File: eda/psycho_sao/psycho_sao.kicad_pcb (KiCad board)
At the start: 2 copper layers, 80.2 x 117.1 mm, 21 parts

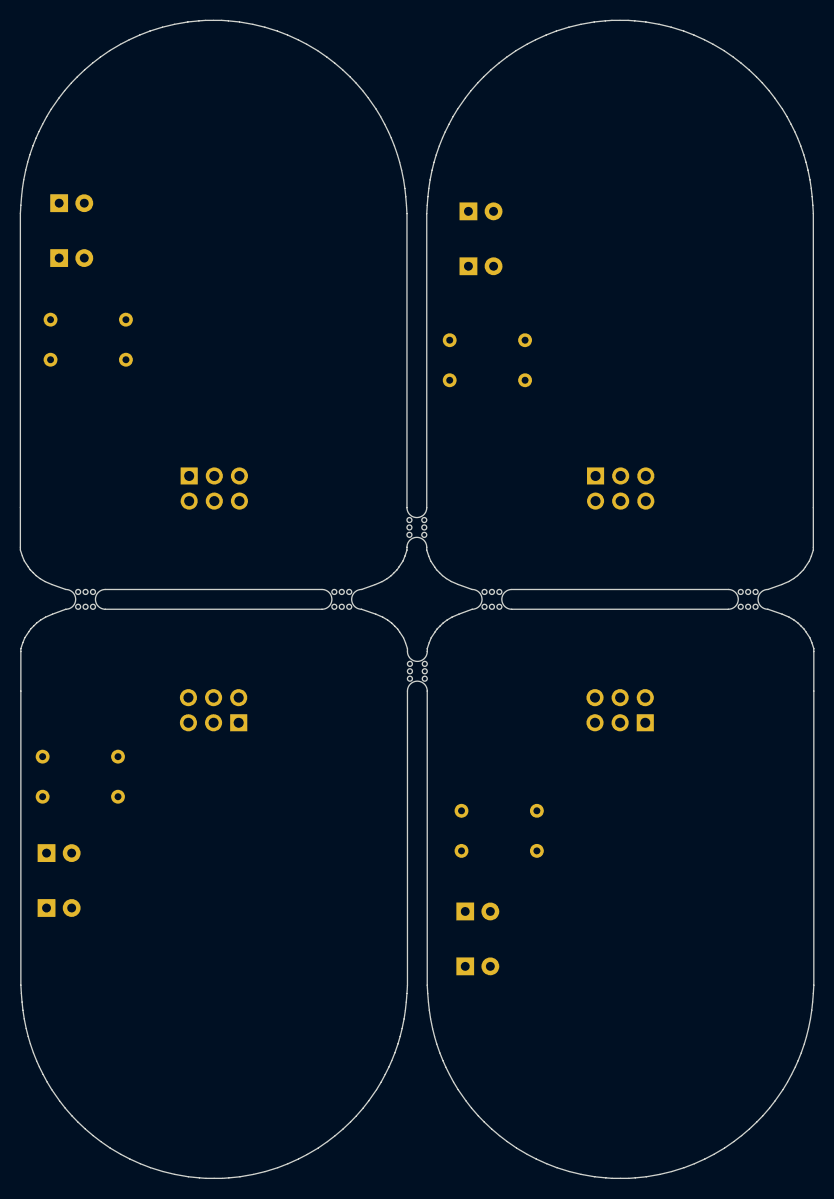
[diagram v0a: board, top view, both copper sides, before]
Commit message: psycho sao scream done
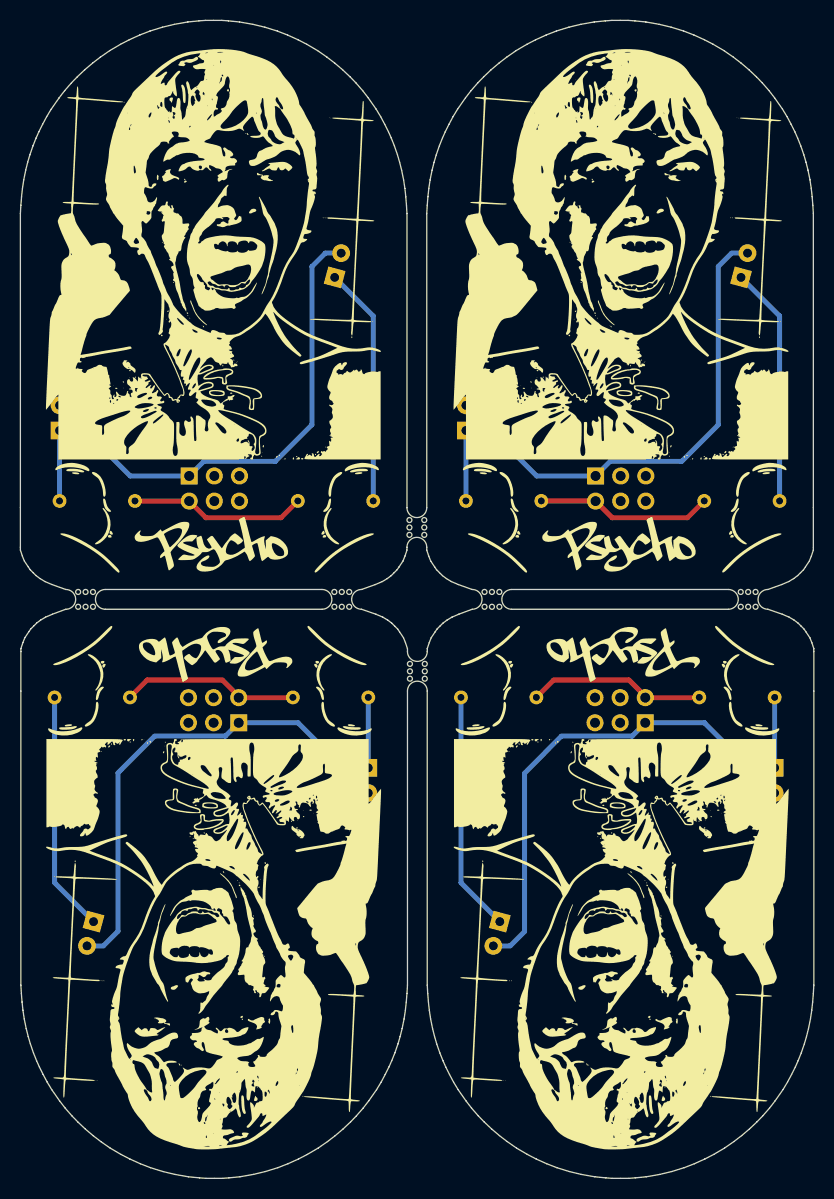
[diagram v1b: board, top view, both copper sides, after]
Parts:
- added Psycho_BMask: Psycho_BMask, 0_badge:Scream_Face_B_Mask, F.Cu at (122.1, 92.7)
- added Psycho_FCu: Psycho_FCu, 0_badge:Scream_Face_F_Cu, F.Cu at (122.1, 92.7)
- added Psycho_FMask: Psycho_FMask, 0_badge:Scream_Face_F_Mask, F.Cu at (122.1, 92.7)
- added Psycho_FSilk: Psycho_FSilk, 0_badge:Scream_Face_F_Silk, F.Cu at (122.1, 92.7)
- JSAO1, JSAO2, JSAO3, JSAO4: footprint 0_sao_v169bis:SAOv169-SAOv3-2x3 -> 0_sao_v169bis:SAOv169-SAOv3-2x3_po
- moved R12 35.6 mm to (116.1, 86.8), turned to 180 degrees
- moved R22 35.5 mm to (157.2, 86.8), turned to 180 degrees
- moved D41 34.5 mm to (156.7, 113.8), turned to -90 degrees
- moved R41 33.7 mm to (156.7, 106.7), turned to 180 degrees
- moved D31 33.6 mm to (115.6, 113.8), turned to -90 degrees
- moved R31 33.5 mm to (115.6, 106.7), turned to 180 degrees
- moved D12 27.9 mm to (112.2, 64.2), turned to 75 degrees
- moved D22 27.6 mm to (153.3, 64.2), turned to 75 degrees
- moved D11 23.0 mm to (84.4, 79.7), turned to 90 degrees
- moved D21 22.2 mm to (125.5, 79.7), turned to 90 degrees
- moved R11 18.3 mm to (84.4, 86.8)
- moved R21 16.3 mm to (125.5, 86.8)
- moved R42 15.5 mm to (125.0, 106.7)
- moved R32 10.1 mm to (83.9, 106.7)
- moved D42 5.72 mm to (128.9, 129.3), turned to -105 degrees
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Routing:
- net +3.3V: track 0.00 -> 50.1 mm
- net +3.3V1: track 0.00 -> 50.1 mm
- net +3.3V3: track 0.00 -> 50.1 mm
- net +3.3V2: track 0.00 -> 50.1 mm
- net Net-(D32-K): track 0.00 -> 24.3 mm
- net Net-(D42-K): track 0.00 -> 24.3 mm
- net Net-(D22-K): track 0.00 -> 24.2 mm
- net Net-(D12-K): track 0.00 -> 24.2 mm
- net GND1: track 0.00 -> 17.9 mm
- net GND: track 0.00 -> 17.9 mm
- net GND2: track 0.00 -> 17.9 mm
- net GND3: track 0.00 -> 17.9 mm
- net Net-(D21-K): track 0.00 -> 7.13 mm
- net Net-(D11-K): track 0.00 -> 7.13 mm
- net Net-(D41-K): track 0.00 -> 7.12 mm
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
